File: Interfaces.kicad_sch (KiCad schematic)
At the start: 14 parts, among them J5 SWD1, J6 I2C1_Headers, J8 UART1_HDR

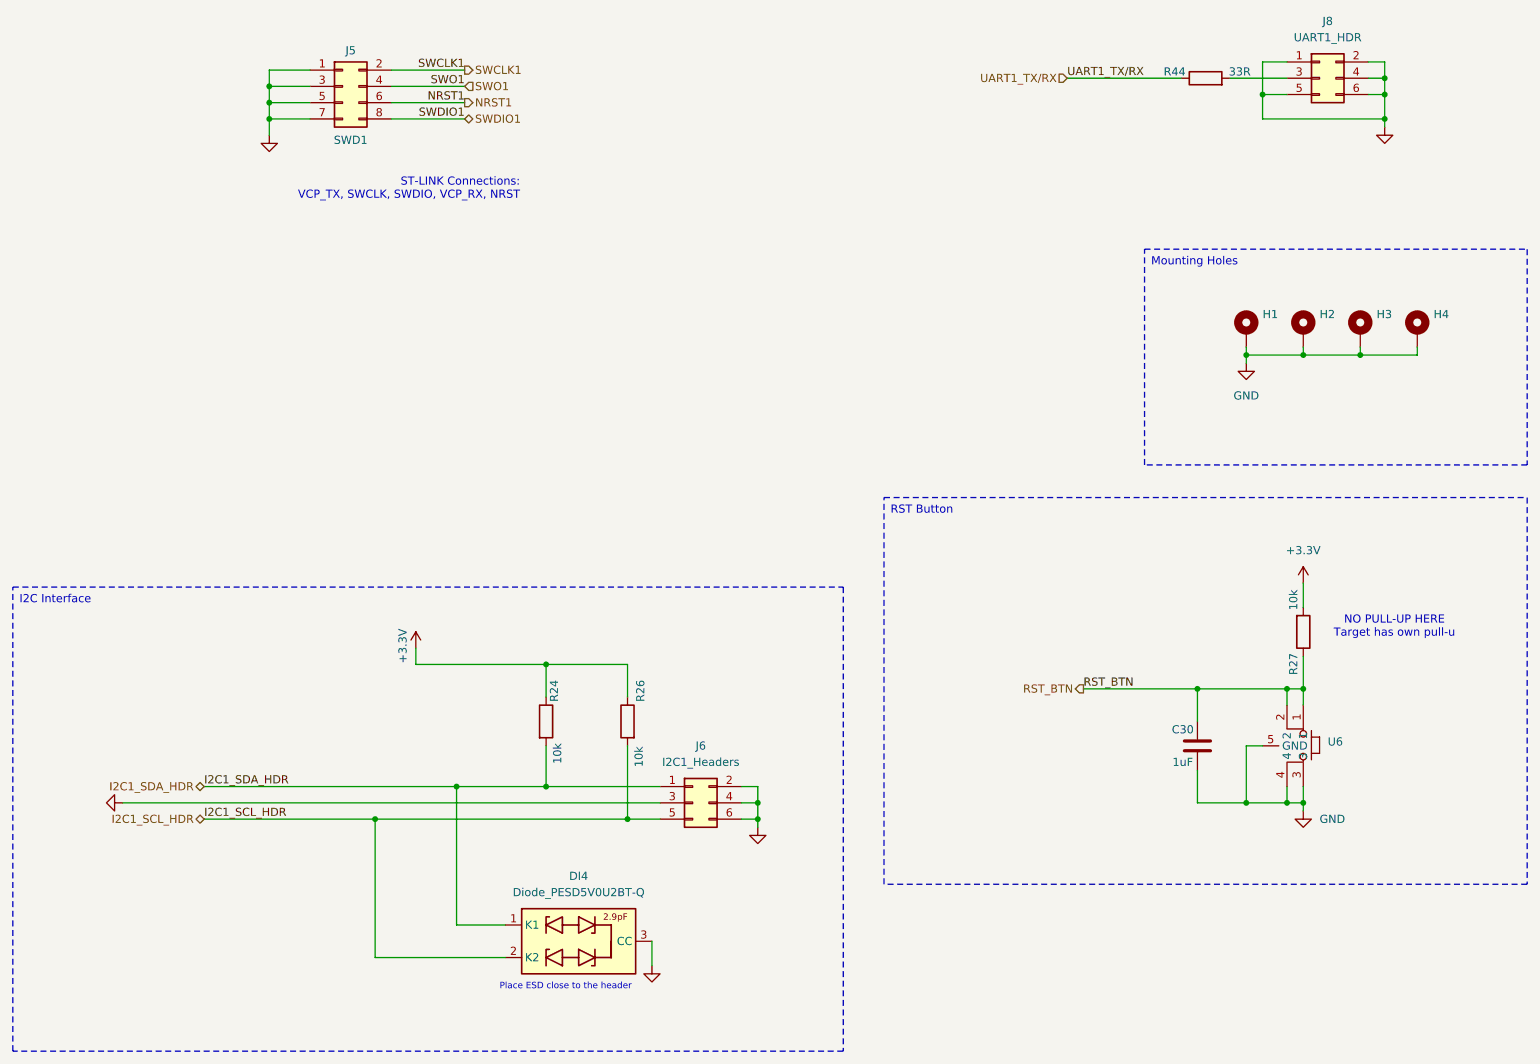
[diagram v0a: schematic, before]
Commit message: Update
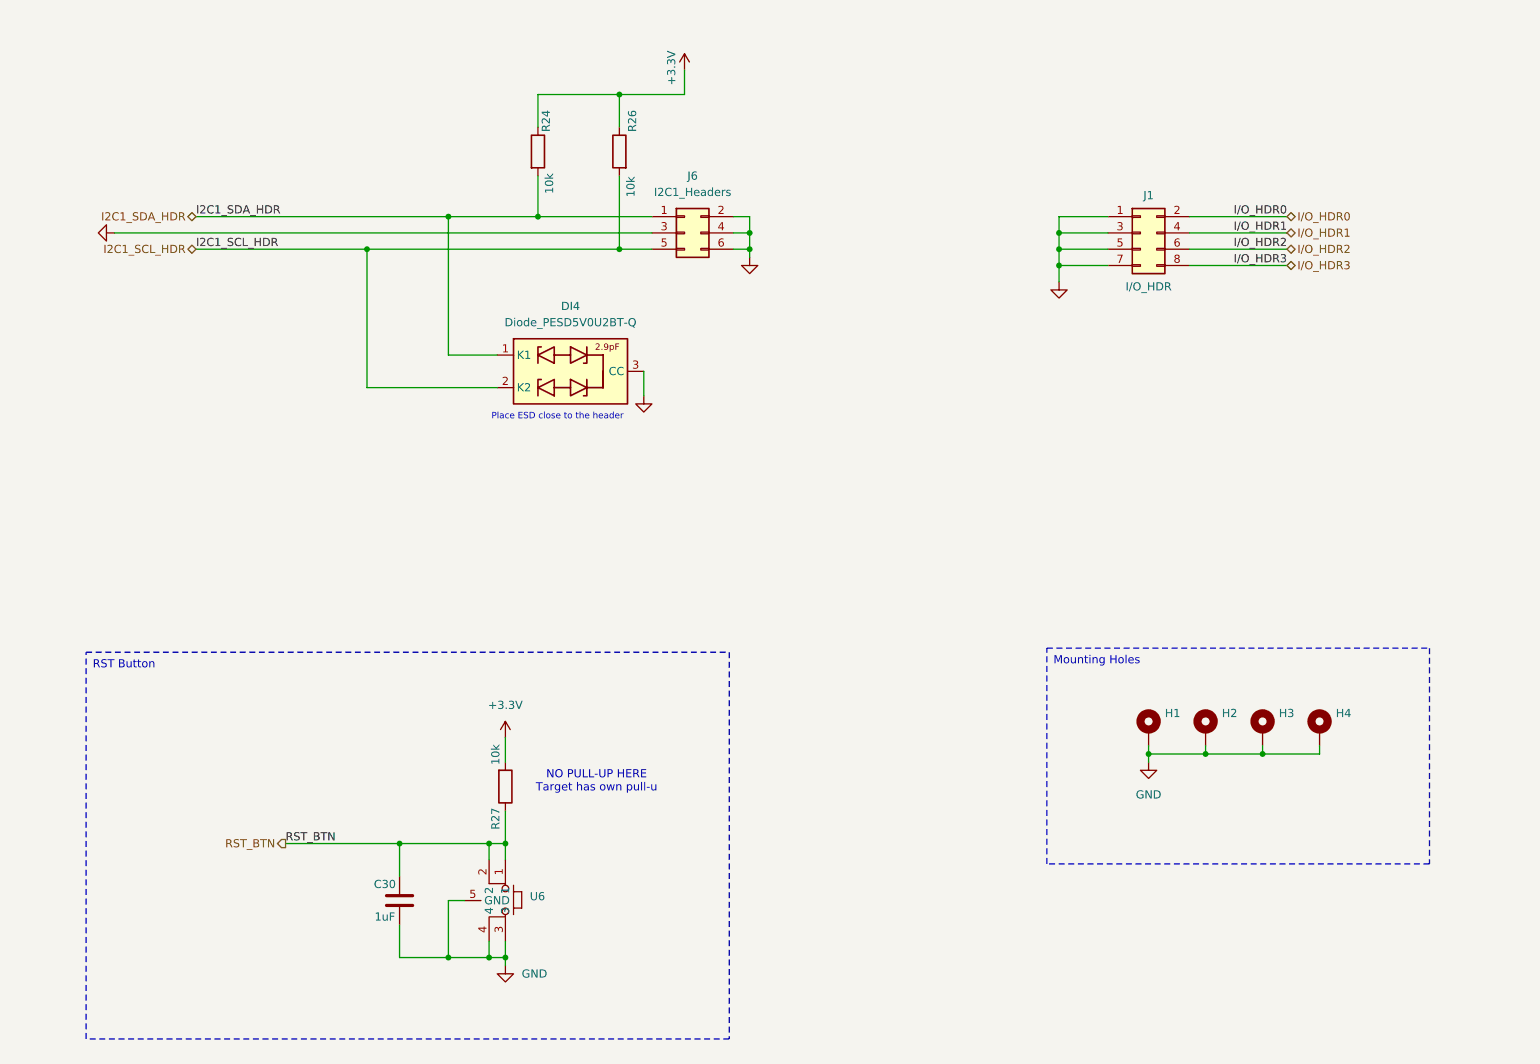
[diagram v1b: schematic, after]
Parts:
- removed J5: SWD1, Connector_PinHeader_2.54mm:PinHeader_2x04_P2.54mm_Horizontal, symbol Connector_Generic:Conn_02x04_Odd_Even
- removed J8: UART1_HDR, Connector_PinHeader_2.54mm:PinHeader_2x03_P2.54mm_Horizontal, symbol Connector_Generic:Conn_02x03_Odd_Even
- removed R44: 33R, Resistor_SMD:R_0805_2012Metric, symbol Device:R
- added J1: I/O_HDR, Connector_PinHeader_2.54mm:PinHeader_2x04_P2.54mm_Horizontal, symbol Connector_Generic:Conn_02x04_Odd_Even
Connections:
- net GND: now also J1.1 (Pin_1), J1.3 (Pin_3), J1.5 (Pin_5), J1.7 (Pin_7)
- new net I/O_HDR0: J1.2 (Pin_2)
- new net I/O_HDR1: J1.4 (Pin_4)
- new net I/O_HDR2: J1.6 (Pin_6)
- new net I/O_HDR3: J1.8 (Pin_8)
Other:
- note removed: "ST-LINK Connections: VCP_TX, SWCLK, SWDIO, VCP_RX, NRST"
- moved on the sheet: C30, DI4, H1, H2, H3, H4, J6, R24, R26, R27, U6
